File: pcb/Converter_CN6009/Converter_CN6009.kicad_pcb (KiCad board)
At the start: 2 copper layers, 45 x 23 mm, 16 parts, among them U1 XL6009

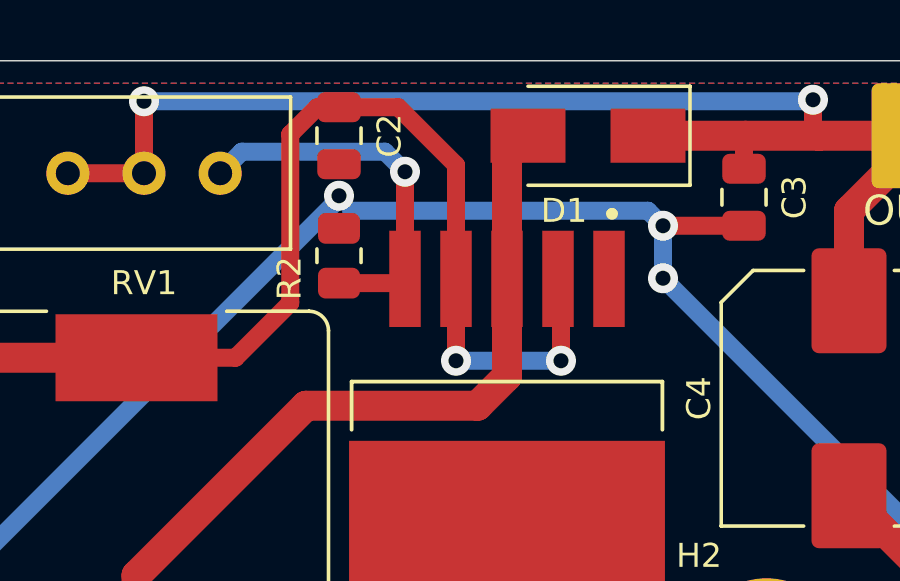
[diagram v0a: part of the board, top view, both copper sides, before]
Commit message: ultima correccion para revision final
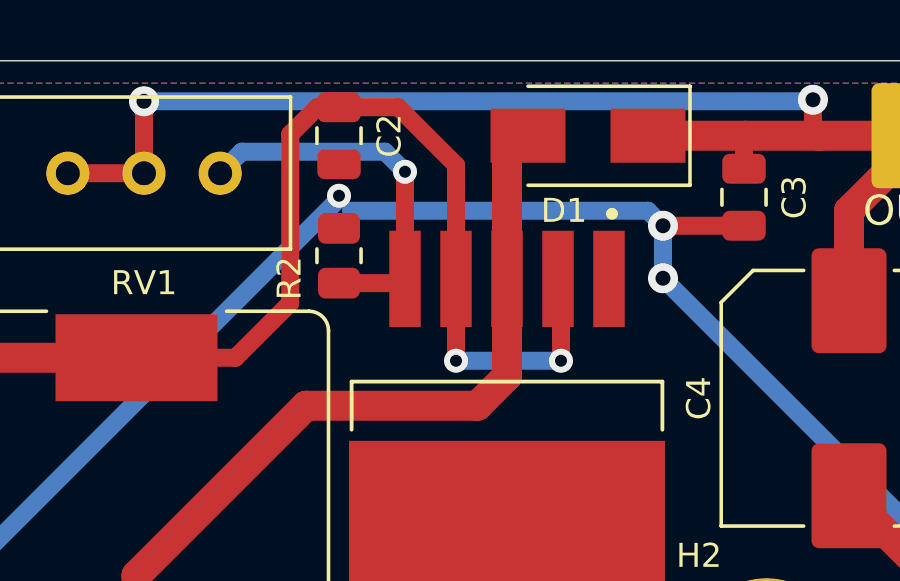
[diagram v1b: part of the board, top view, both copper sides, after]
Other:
- board text added: "* 0,4 mm agujero de via"
- board text added: "* 0,8 mm pad de via"
